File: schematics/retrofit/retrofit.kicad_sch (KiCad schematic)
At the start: 0 parts

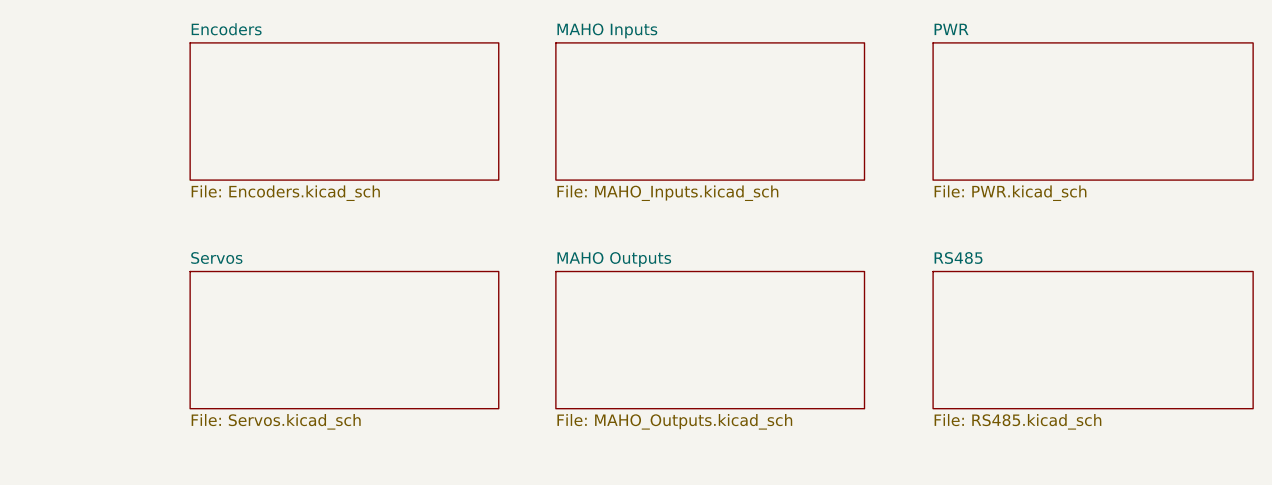
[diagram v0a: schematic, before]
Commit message: schematics
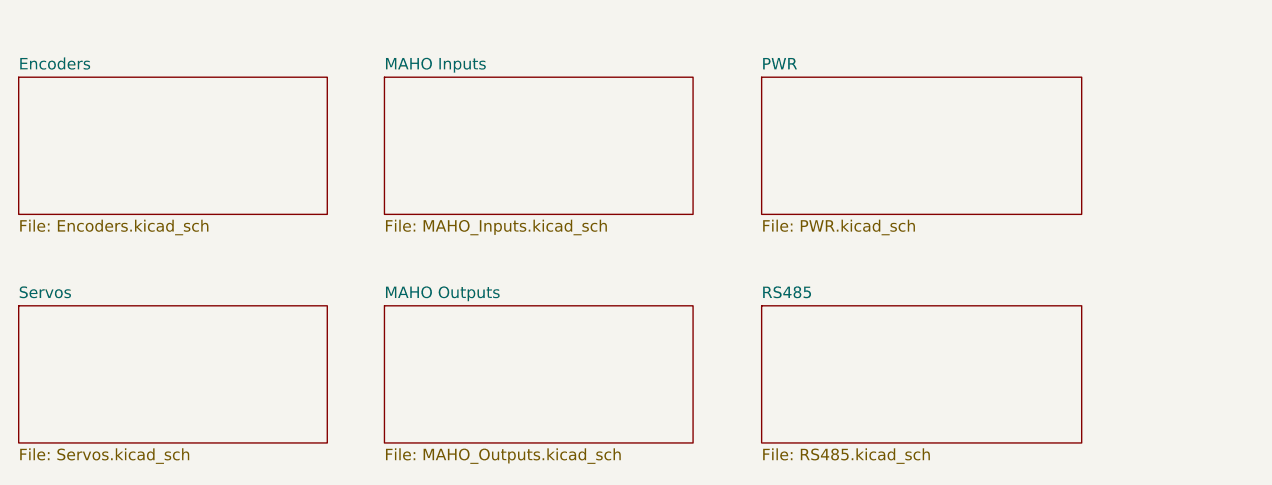
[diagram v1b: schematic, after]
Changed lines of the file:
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@@
 (kicad_sch (version 20230121) (generator eeschema)
   (paper "A4")
-  (sheet (at 186.69 69.85) (size 35.56 15.24) (fields_autoplaced)
+  (sheet (at 167.64 73.66) (size 35.56 15.24) (fields_autoplaced)
     (stroke (width 0.1524) (type solid))
     (fill (color 0 0 0 0.0000))
-    (property "Sheetname" "PWR" (at 186.69 69.1384 0)
+    (property "Sheetname" "PWR" (at 167.64 72.9484 0)
       (effects (font (size 1.27 1.27)) (justify left bottom))
     )
-    (property "Sheetfile" "PWR.kicad_sch" (at 186.69 85.6746 0)
+    (property "Sheetfile" "PWR.kicad_sch" (at 167.64 89.4846 0)
       (effects (font (size 1.27 1.27)) (justify left top))
     )
@@
     )
   )
-  (sheet (at 144.78 69.85) (size 34.29 15.24) (fields_autoplaced)
+  (sheet (at 125.73 73.66) (size 34.29 15.24) (fields_autoplaced)
     (stroke (width 0.1524) (type solid))
     (fill (color 0 0 0 0.0000))
-    (property "Sheetname" "MAHO Inputs" (at 144.78 69.1384 0)
+    (property "Sheetname" "MAHO Inputs" (at 125.73 72.9484 0)
       (effects (font (size 1.27 1.27)) (justify left bottom))
     )
-    (property "Sheetfile" "MAHO_Inputs.kicad_sch" (at 144.78 85.6746 0)
+    (property "Sheetfile" "MAHO_Inputs.kicad_sch" (at 125.73 89.4846 0)
       (effects (font (size 1.27 1.27)) (justify left top))
     )
@@
     )
   )
-  (sheet (at 104.14 95.25) (size 34.29 15.24) (fields_autoplaced)
+  (sheet (at 85.09 99.06) (size 34.29 15.24) (fields_autoplaced)
     (stroke (width 0.1524) (type solid))
     (fill (color 0 0 0 0.0000))
-    (property "Sheetname" "Servos" (at 104.14 94.5384 0)
+    (property "Sheetname" "Servos" (at 85.09 98.3484 0)
       (effects (font (size 1.27 1.27)) (justify left bottom))
     )
-    (property "Sheetfile" "Servos.kicad_sch" (at 104.14 111.0746 0)
+    (property "Sheetfile" "Servos.kicad_sch" (at 85.09 114.8846 0)
       (effects (font (size 1.27 1.27)) (justify left top))
     )
@@
     )
   )
-  (sheet (at 186.69 95.25) (size 35.56 15.24) (fields_autoplaced)
+  (sheet (at 167.64 99.06) (size 35.56 15.24) (fields_autoplaced)
     (stroke (width 0.1524) (type solid))
     (fill (color 0 0 0 0.0000))
-    (property "Sheetname" "RS485" (at 186.69 94.5384 0)
+    (property "Sheetname" "RS485" (at 167.64 98.3484 0)
       (effects (font (size 1.27 1.27)) (justify left bottom))
     )
-    (property "Sheetfile" "RS485.kicad_sch" (at 186.69 111.0746 0)
+    (property "Sheetfile" "RS485.kicad_sch" (at 167.64 114.8846 0)
       (effects (font (size 1.27 1.27)) (justify left top))
     )
@@
     )
   )
-  (sheet (at 144.78 95.25) (size 34.29 15.24) (fields_autoplaced)
+  (sheet (at 125.73 99.06) (size 34.29 15.24) (fields_autoplaced)
     (stroke (width 0.1524) (type solid))
     (fill (color 0 0 0 0.0000))
-    (property "Sheetname" "MAHO Outputs" (at 144.78 94.5384 0)
+    (property "Sheetname" "MAHO Outputs" (at 125.73 98.3484 0)
       (effects (font (size 1.27 1.27)) (justify left bottom))
     )
-    (property "Sheetfile" "MAHO_Outputs.kicad_sch" (at 144.78 111.0746 0)
+    (property "Sheetfile" "MAHO_Outputs.kicad_sch" (at 125.73 114.8846 0)
       (effects (font (size 1.27 1.27)) (justify left top))
     )
@@
     )
   )
-  (sheet (at 104.14 69.85) (size 34.29 15.24) (fields_autoplaced)
+  (sheet (at 85.09 73.66) (size 34.29 15.24) (fields_autoplaced)
     (stroke (width 0.1524) (type solid))
     (fill (color 0 0 0 0.0000))
-    (property "Sheetname" "Encoders" (at 104.14 69.1384 0)
+    (property "Sheetname" "Encoders" (at 85.09 72.9484 0)
       (effects (font (size 1.27 1.27)) (justify left bottom))
     )
-    (property "Sheetfile" "Encoders.kicad_sch" (at 104.14 85.6746 0)
+    (property "Sheetfile" "Encoders.kicad_sch" (at 85.09 89.4846 0)
       (effects (font (size 1.27 1.27)) (justify left top))
     )
